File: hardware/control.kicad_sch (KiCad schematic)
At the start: 8 parts, among them U1 STM32G0C1KCTxN

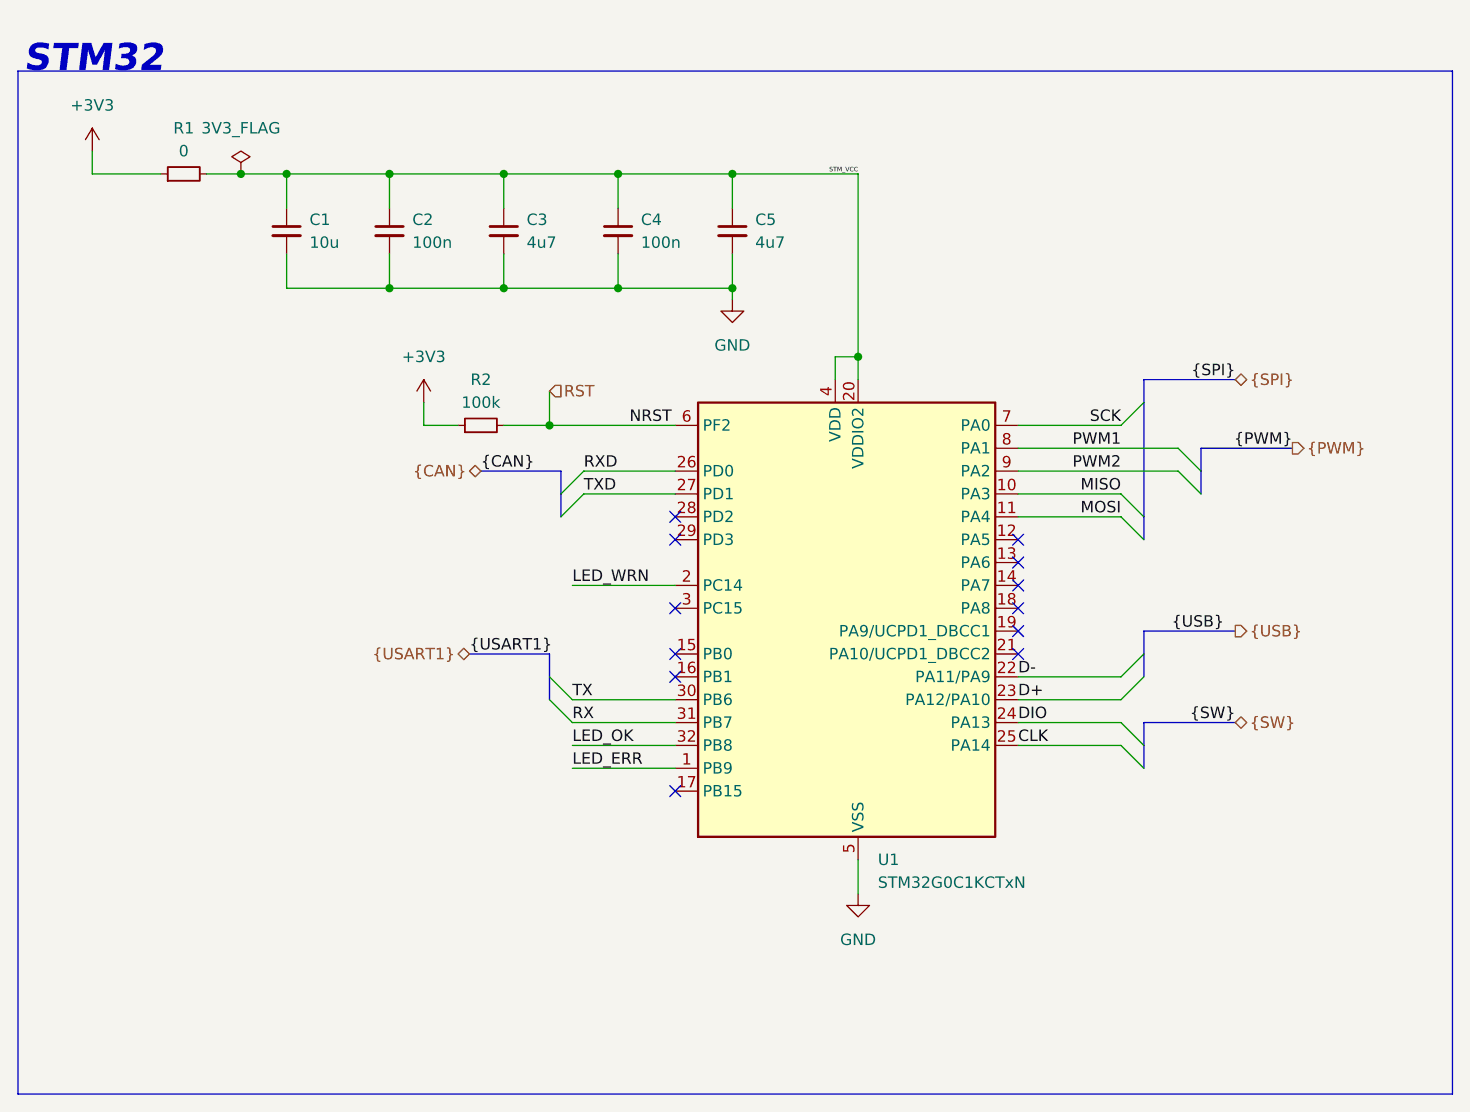
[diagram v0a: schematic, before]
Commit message: schematic & pcb update
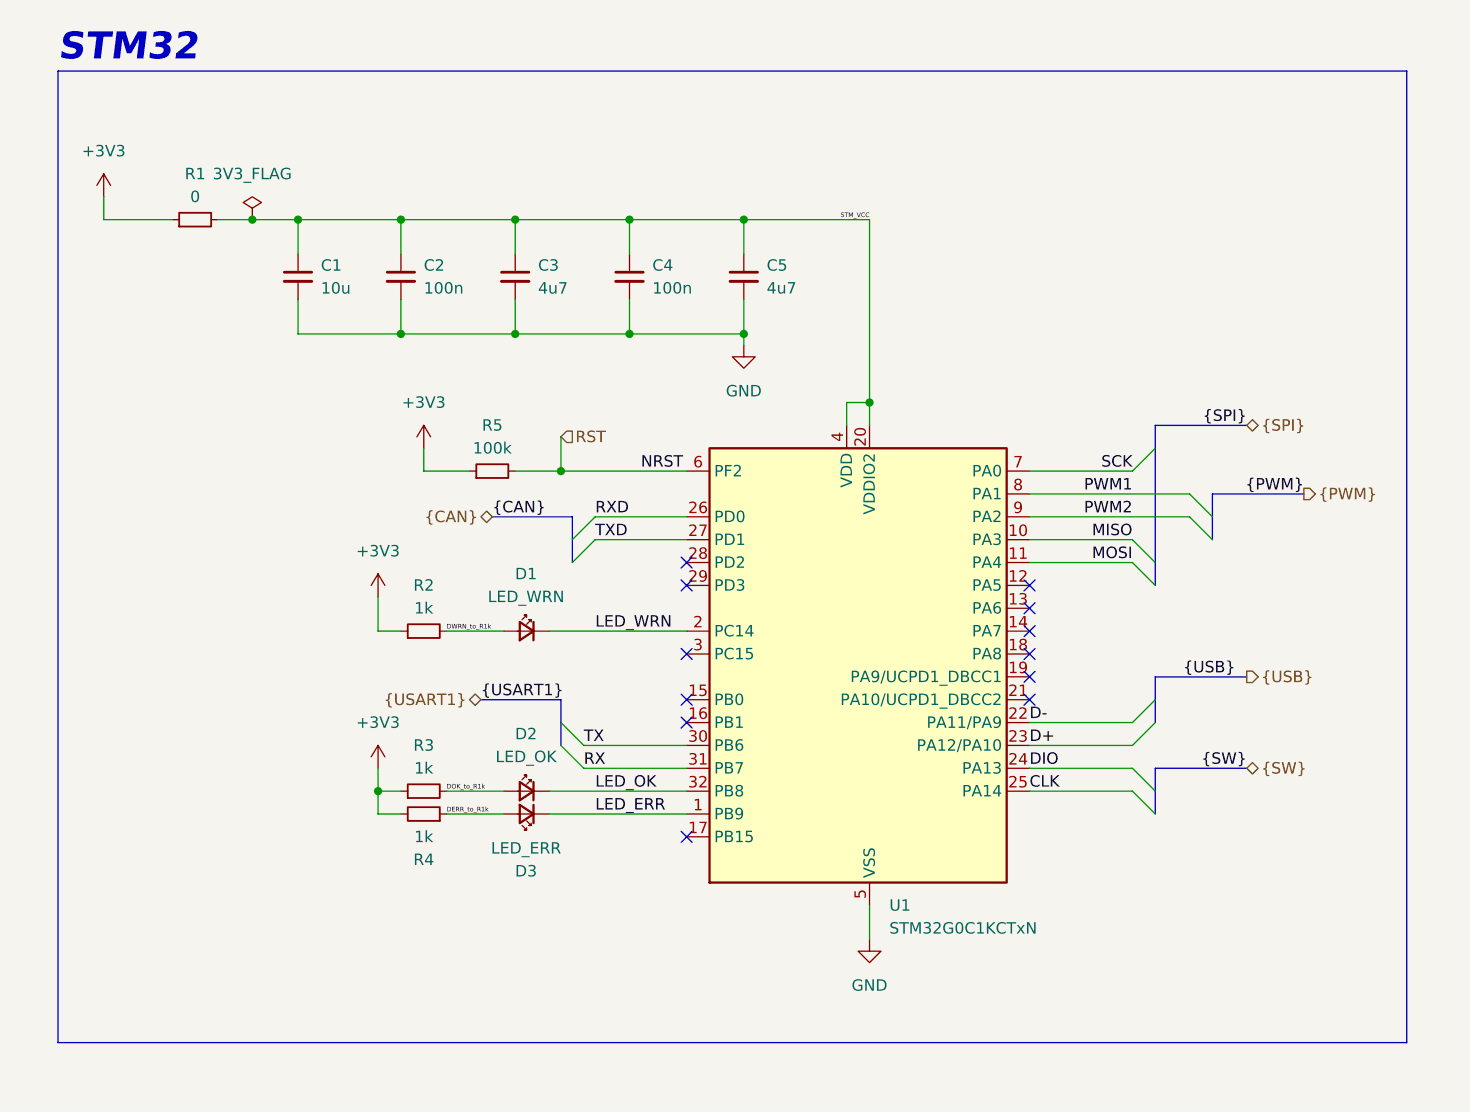
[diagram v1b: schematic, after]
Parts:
- added D1: LED_WRN, LED_SMD:LED_0603_1608Metric, symbol Device:LED_Small
- added D2: LED_OK, LED_SMD:LED_0603_1608Metric, symbol Device:LED_Small
- added D3: LED_ERR, LED_SMD:LED_0603_1608Metric, symbol Device:LED_Small
- added R2, R3, R4: 1k, Resistor_SMD:R_0603_1608Metric_Pad0.98x0.95mm_HandSolder, symbol Device:R_Small
- renumbered R2 to R5
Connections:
- net +3V3: now also R2.1, R3.1, R4.2
- net LED_ERR: now also D3.1 (K)
- net LED_OK: now also D2.1 (K)
- net LED_WRN: now also D1.1 (K)
- new net DERR_to_R1k: D3.2 (A), R4.1
- new net DOK_to_R1k: D2.2 (A), R3.2
- new net DWRN_to_R1k: D1.2 (A), R2.2
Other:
- moved on the sheet: C1, C2, C3, C4, C5, R1, R5, U1
